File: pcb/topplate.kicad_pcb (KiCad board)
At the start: 2 copper layers, 128.6 x 95.2 mm, 28 parts, among them SW1 SW_PUSH, SW10 SW_PUSH, SW11 SW_PUSH, SW12 SW_PUSH, SW13 SW_PUSH, SW14 SW_PUSH, SW15 SW_PUSH, SW16 SW_PUSH, SW17 SW_PUSH, SW18 SW_PUSH, SW19 SW_PUSH, SW2 SW_PUSH, SW20 SW_PUSH, SW21 SW_PUSH, SW3 SW_PUSH, SW4 SW_PUSH, SW5 SW_PUSH, SW6 SW_PUSH, SW7 SW_PUSH, SW8 SW_PUSH, SW9 SW_PUSH

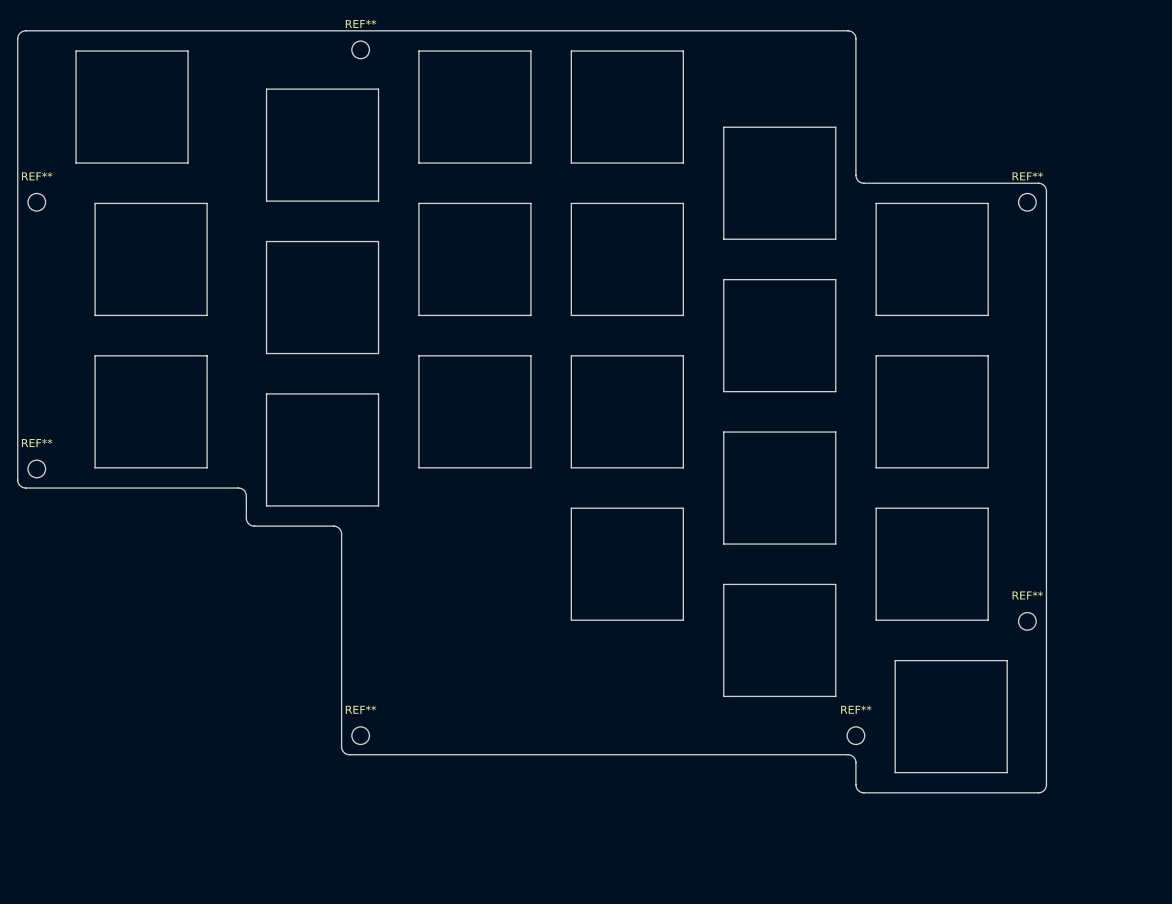
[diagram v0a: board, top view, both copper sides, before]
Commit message: add: pcb and plate garber files
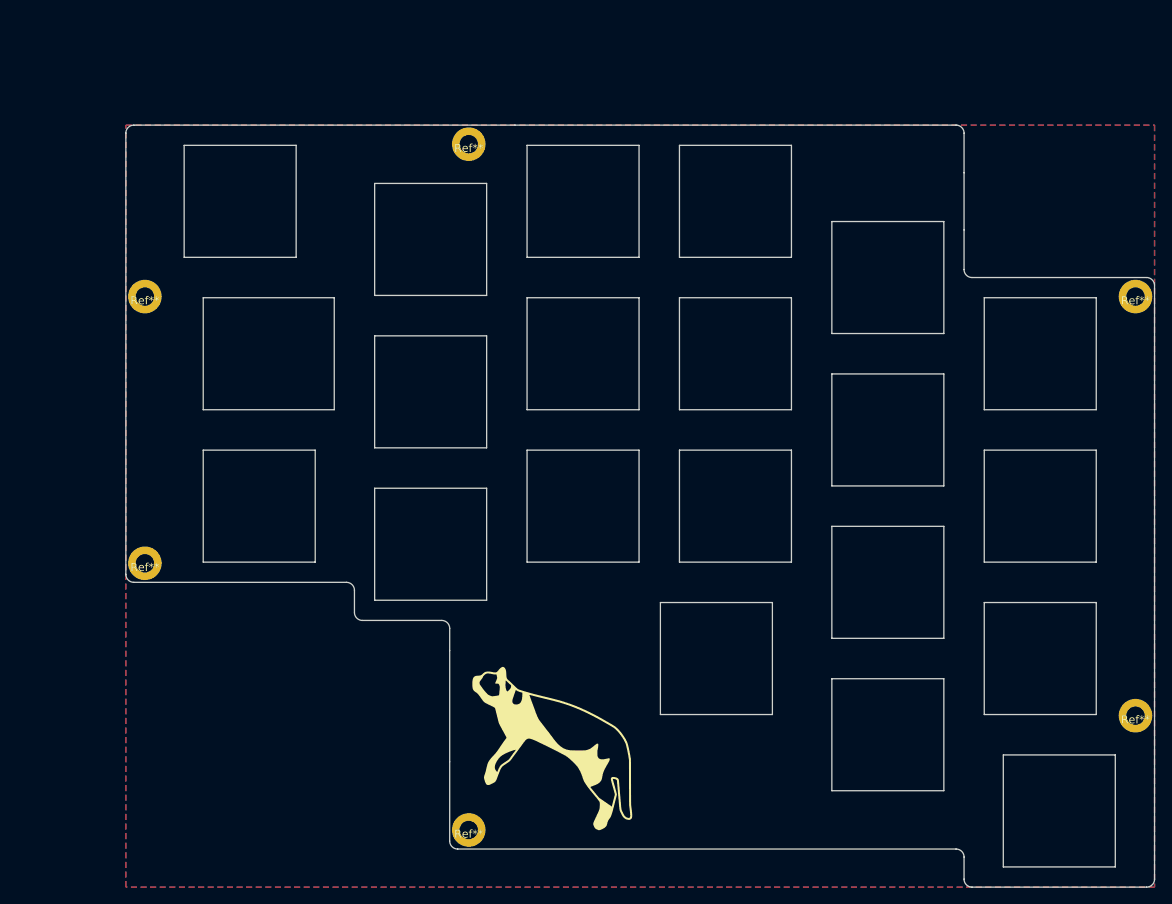
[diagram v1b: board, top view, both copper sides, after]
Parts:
- removed REF** (x7): MountingHole_2.2mm_M2, MountingHole:MountingHole_2.2mm_M2
- added G***: LOGO, maggie:maggie_reverse, F.Cu at (81.1, 104.0)
- added Ref**: Val**, kbd:M2_Hole_TH, F.Cu at (70.7, 28.5)
- added Ref**: Val**, kbd:M2_Hole_TH, F.Cu at (154.0, 47.5)
- added Ref**: Val**, kbd:M2_Hole_TH, F.Cu at (30.2, 47.5)
- added Ref**: Val**, kbd:M2_Hole_TH, F.Cu at (154.0, 99.9)
- added Ref**: Val**, kbd:M2_Hole_TH, F.Cu at (70.7, 114.2)
- added Ref**: Val**, kbd:M2_Hole_TH, F.Cu at (30.2, 80.8)
- SW7: footprint kbd:SW_Hole -> kbd:SW_Hole_1+1.25
- moved SW7 18.8 mm to (45.7, 54.6)
- moved SW14 17.9 mm to (65.9, 78.5)
- moved SW20 17.9 mm to (123.0, 102.3)
- moved SW10 17.9 mm to (104.0, 54.6)
- moved SW15 17.9 mm to (85.0, 73.7)
- moved SW16 17.9 mm to (104.0, 73.7)
- moved SW2 17.9 mm to (65.9, 40.4)
- moved SW3 17.9 mm to (85.0, 35.6)
- moved SW4 17.9 mm to (104.0, 35.6)
- moved SW5 17.9 mm to (123.0, 45.1)
- moved SW8 17.9 mm to (65.9, 59.4)
- moved SW9 17.9 mm to (85.0, 54.6)
- moved SW1 17.9 mm to (42.1, 35.6)
- moved SW13 17.9 mm to (44.5, 73.7)
- moved SW11 17.9 mm to (123.0, 64.2)
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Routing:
- added copper zone on B.Cu, net GND
- added copper zone on F.Cu, net GND
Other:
- outline, holes or cut-outs redrawn
- board text added: "Maggie42cs Studio Purring"
